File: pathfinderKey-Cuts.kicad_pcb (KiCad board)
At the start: 2 copper layers, 78 x 60.5 mm, 13 parts, among them SW1 SW_Push, SW2 SW_Push, SW3 SW_Push, SW4 SW_Push, U1 XIAO-RP2040-DIP

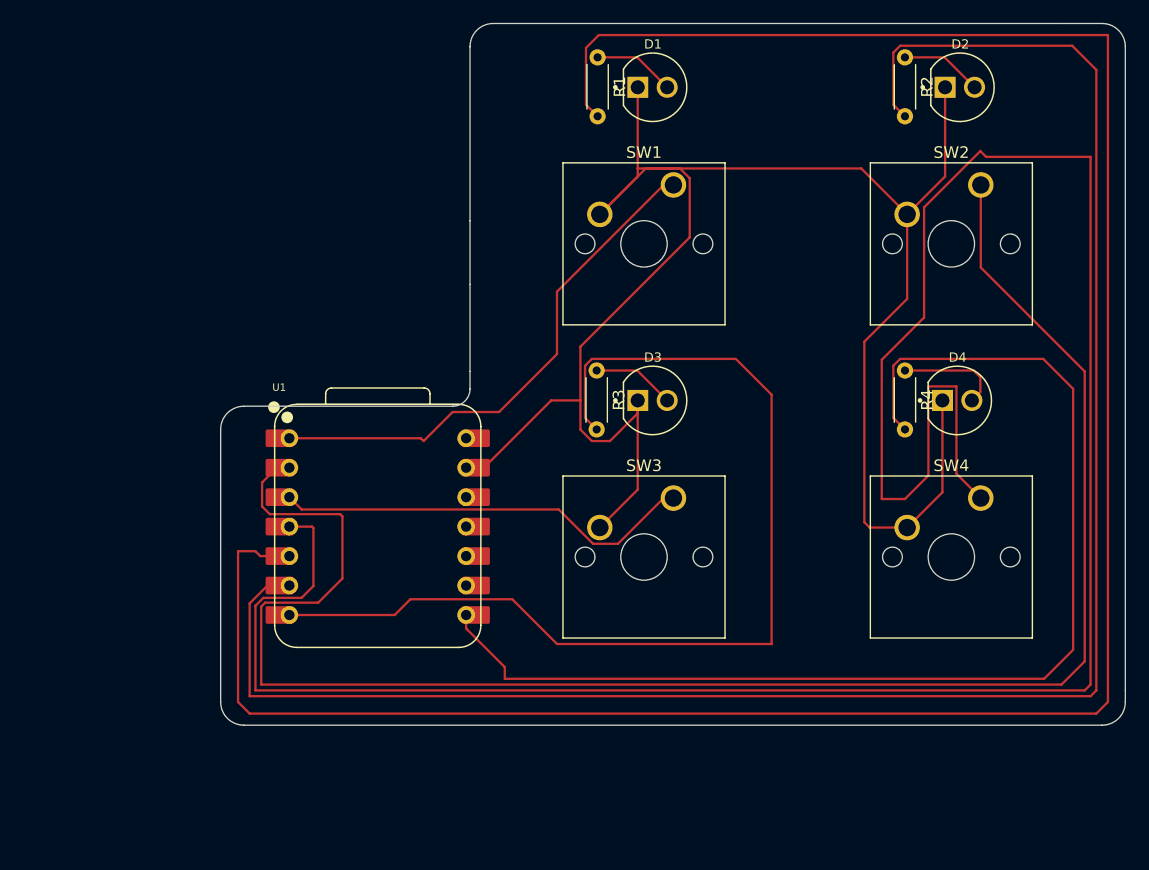
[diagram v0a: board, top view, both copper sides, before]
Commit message: Add files via upload
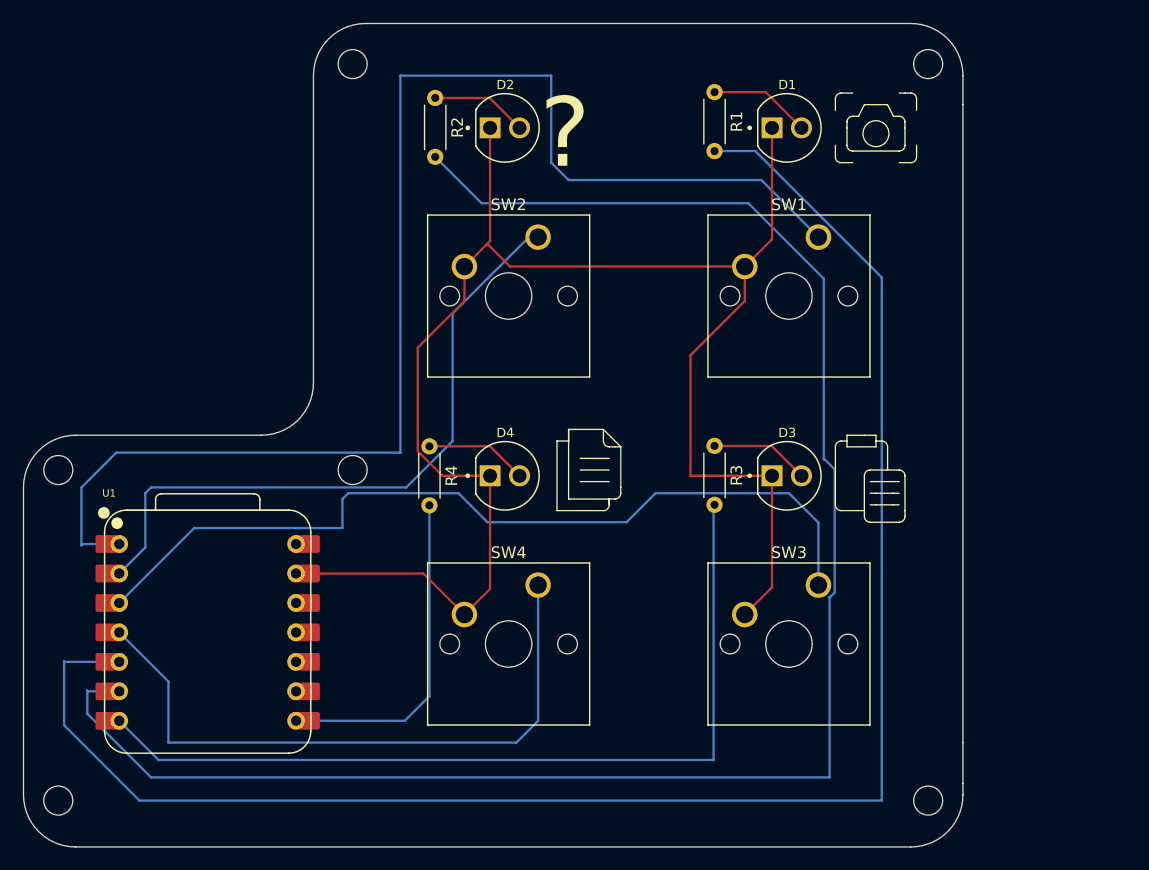
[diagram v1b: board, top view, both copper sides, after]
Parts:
- moved R4 41.5 mm to (154.0, 114.5)
- moved R2 40.7 mm to (154.5, 84.4)
- moved D4 39.5 mm to (160.5, 117.0)
- moved D2 39.4 mm to (160.5, 87.0)
- moved SW4 38.9 mm to (163.4, 126.4)
- moved SW2 38.4 mm to (163.4, 96.4)
- moved U1 17.3 mm to (134.9, 130.5)
- moved SW3 14.6 mm to (187.5, 126.4)
- moved SW1 13.3 mm to (187.5, 96.4)
- moved D3 13.3 mm to (184.8, 117.0)
- moved D1 12.1 mm to (184.8, 87.0)
- moved R3 12.1 mm to (178.6, 114.4)
- moved R1 10.5 mm to (178.6, 83.9)
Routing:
- net button4: track 206.5 -> 55.6 mm
- net button2: track 149.7 -> 57.3 mm
- net LED4: track 102.1 -> 28.8 mm
- net button1: track 45.5 -> 115.8 mm
- net LED1: track 202.7 -> 147.5 mm
- net button3: track 36.4 -> 74.2 mm
- net GND: track 161.7 -> 142.3 mm
- net LED3: track 88.7 -> 74.7 mm
- net LED2: track 163.3 -> 152.7 mm
- net Net-(D1-PadA): track 7.07 -> 8.78 mm
- net Net-(D3-PadA): track 7.15 -> 8.57 mm
- net Net-(D2-PadA): track 7.07 -> 8.34 mm
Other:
- board size 78 x 60.5 mm -> 81 x 71 mm
- board text added: "?"
